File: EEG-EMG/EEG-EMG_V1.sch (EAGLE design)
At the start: 63 parts, among them IC1 MCP6V31, IC11 LM7332MA, IC2 MCP6V31, IC3 MCP6V31, IC4 MCP6V31, IC6 MCP3912, Q7 CSM-3X-CRYSTALCSM-3X, U2 BGM111-VISUAL-A

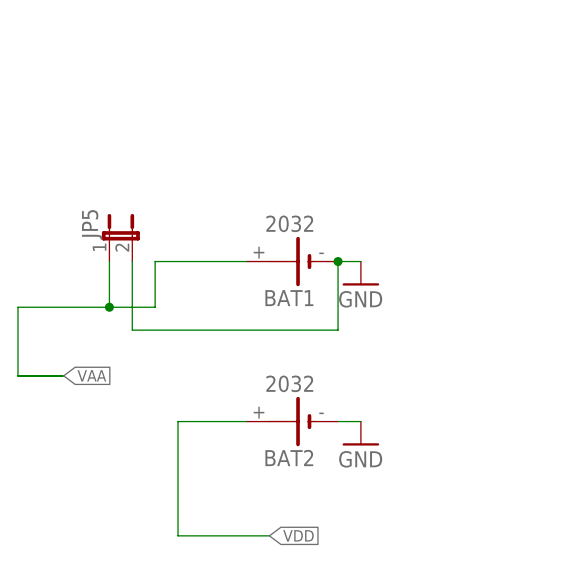
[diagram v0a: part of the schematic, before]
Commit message: Completed Board
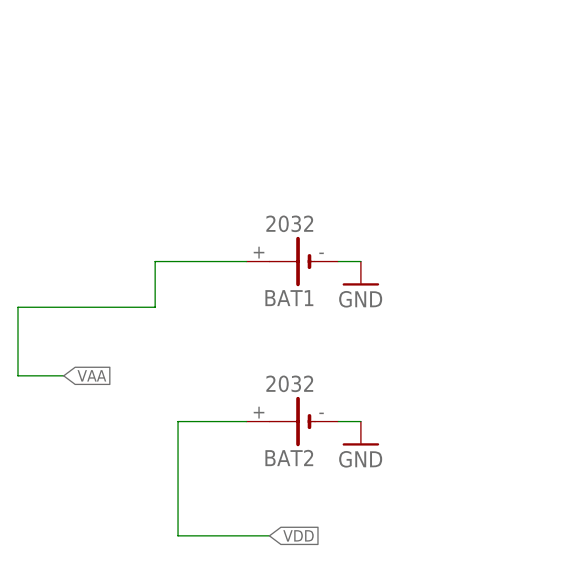
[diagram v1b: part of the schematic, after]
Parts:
- removed JP5: (no value), jumper:JP1E
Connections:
- net GND: no longer JP5.2
- net VAA: no longer JP5.1
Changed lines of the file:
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@@
 <part name="GND29" library="SparkFun-Aesthetics" deviceset="GND" device=""/>
 <part name="J2" library="tag-connect" deviceset="TC2030" device="-MCP-NL"/>
-<part name="JP5" library="jumper" deviceset="JP1E" device=""/>
 </parts>
 <sheets>
@@
 <instance part="GND29" gate="1" x="1013.46" y="-233.68"/>
 <instance part="J2" gate="G$1" x="982.98" y="-228.6" rot="R180"/>
-<instance part="JP5" gate="A" x="360.68" y="-40.64"/>
 </instances>
 <busses>
@@
 <wire x1="386.08" y1="-43.18" x2="388.62" y2="-43.18" width="0.1524" layer="91"/>
 <pinref part="BAT1" gate="G$1" pin="-"/>
-<pinref part="JP5" gate="A" pin="2"/>
-<wire x1="363.22" y1="-43.18" x2="363.22" y2="-50.8" width="0.1524" layer="91"/>
-<wire x1="363.22" y1="-50.8" x2="386.08" y2="-50.8" width="0.1524" layer="91"/>
-<wire x1="386.08" y1="-50.8" x2="386.08" y2="-43.18" width="0.1524" layer="91"/>
-<junction x="386.08" y="-43.18"/>
 </segment>
 <segment>
@@
 <wire x1="365.76" y1="-43.18" x2="375.92" y2="-43.18" width="0.1524" layer="91"/>
 <pinref part="BAT1" gate="G$1" pin="+"/>
-<pinref part="JP5" gate="A" pin="1"/>
-<wire x1="360.68" y1="-43.18" x2="360.68" y2="-48.26" width="0.1524" layer="91"/>
-<wire x1="360.68" y1="-48.26" x2="365.76" y2="-48.26" width="0.1524" layer="91"/>
 <wire x1="365.76" y1="-48.26" x2="365.76" y2="-43.18" width="0.1524" layer="91"/>
 <wire x1="350.52" y1="-48.26" x2="350.52" y2="-55.88" width="0.1524" layer="91"/>
-<wire x1="350.52" y1="-55.88" x2="355.6" y2="-55.88" width="0.1524" layer="91"/>
 <label x="355.6" y="-55.88" size="1.27" layer="95" xref="yes"/>
-<wire x1="360.68" y1="-48.26" x2="350.52" y2="-48.26" width="0.1524" layer="91"/>
-<junction x="360.68" y="-48.26"/>
+<wire x1="365.76" y1="-48.26" x2="350.52" y2="-48.26" width="0.1524" layer="91"/>
 <label x="558.8" y="5.08" size="1.27" layer="95" xref="yes"/>
 <wire x1="350.52" y1="-55.88" x2="355.6" y2="-55.88" width="0.1524" layer="91"/>
-<wire x1="350.52" y1="-55.88" x2="355.6" y2="-55.88" width="0.1524" layer="91"/>
 <label x="637.54" y="-25.4" size="1.27" layer="95" xref="yes"/>
